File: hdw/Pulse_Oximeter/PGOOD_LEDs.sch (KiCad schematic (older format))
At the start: 8 parts

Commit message: Continued schematic development
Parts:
- removed C?: 0.1uF, Capacitors_SMD:C_0402, symbol Custom_Library:C_Custom
- removed D?: Green, LEDs:LED_0402, symbol Device:LED
- removed R?: 1k, Resistors_SMD:R_0402, symbol Custom_Library:R_Custom
- removed U?: 74LVC1G97, Package_TO_SOT_SMD:SOT-363_SC-70-6, symbol Custom_Library:74LVC1G97_Power_NOT
- added C? (x4): 0.1uF, Capacitors_SMD:C_0603, symbol Custom_Library:C_Custom
- added C?: 4.7uF, Capacitors_SMD:C_0805, symbol Custom_Library:C_Custom
- added D? (x4): Green, LEDs:LED_0603, symbol Device:LED
- added R? (x4): 1k, Resistors_SMD:R_0603, symbol Custom_Library:R_Custom
- added U? (x4): 74LVC1G97, Package_TO_SOT_SMD:SOT-363_SC-70-6, symbol Custom_Library:74LVC1G97_Power_NOT
- added U?: TPS71533, Package_TO_SOT_SMD:SOT-353_SC-70-5, symbol Regulator_Linear:TPS71533__SC70
- C?: footprint Capacitors_SMD:C_0402 -> Capacitors_SMD:C_0603; Digi-Key PN 490-10701-1-ND -> 311-1344-1-ND; display_footprint 0402 -> 0603
- D?: footprint LEDs:LED_0402 -> LEDs:LED_0603; Digi-Key PN 1497-1219-1-ND -> 160-1446-1-ND
- R?: footprint Resistors_SMD:R_0402 -> Resistors_SMD:R_0603; Digi-Key PN 541-1.00KLCT-ND -> RMCF0603FT1K00CT-ND; Wattage 1/16W -> 1/10W; display_footprint 0402 -> 0603
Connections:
- net labels added: +12V, POS12_PGOOD, POS1P8_PGOOD
- net labels removed: +5V_USB, GND_USB
- wire segments 4 -> 19
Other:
- moved on the sheet: C?, D?, R?

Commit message: Added display circuits
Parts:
- removed U? (x5): 74LVC1G97, Package_TO_SOT_SMD:SOT-363_SC-70-6, symbol Custom_Library:74LVC1G97_Power_NOT
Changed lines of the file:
@@
 EESchema Schematic File Version 4
+LIBS:Pulse_Oximeter-cache
 EELAYER 30 0
 EELAYER END
@@
 POS5_USB_PGOOD
 $Comp
-L Custom_Library:74LVC1G97_Power_NOT U?
-U 1 1 5E4A38CE
-P 4980 2870
-AR Path="/5CB7A8BC/5E4A38CE" Ref="U?"  Part="1"
-AR Path="/5CB7A8C3/5E4A38CE" Ref="U?"  Part="1"
-AR Path="/5EAE4ADE/5E4A38CE" Ref="U?"  Part="1"
-F 0 "U?" H 5040 3020 50  0000 L CNN
-F 1 "74LVC1G97" H 5040 2720 50  0000 L CNN
-F 2 "Package_TO_SOT_SMD:SOT-363_SC-70-6" H 5030 2870 50  0001 C CNN
-F 3 "http://www.ti.com/lit/ds/symlink/sn74lvc1g97.pdf" H 5030 2870 50  0001 C CNN
-F 4 "296-15582-1-ND" H 4980 2870 50  0001 C CNN "Digi-Key PN"
-	1    4980 2870
-	1    0    0    -1
-$EndComp
-$Comp
-L Custom_Library:74LVC1G97_Power_NOT U?
-U 1 1 5E4A4421
-P 6980 2870
-AR Path="/5CB7A8BC/5E4A4421" Ref="U?"  Part="1"
-AR Path="/5CB7A8C3/5E4A4421" Ref="U?"  Part="1"
-AR Path="/5EAE4ADE/5E4A4421" Ref="U?"  Part="1"
-F 0 "U?" H 7040 3020 50  0000 L CNN
-F 1 "74LVC1G97" H 7040 2720 50  0000 L CNN
-F 2 "Package_TO_SOT_SMD:SOT-363_SC-70-6" H 7030 2870 50  0001 C CNN
-F 3 "http://www.ti.com/lit/ds/symlink/sn74lvc1g97.pdf" H 7030 2870 50  0001 C CNN
-F 4 "296-15582-1-ND" H 6980 2870 50  0001 C CNN "Digi-Key PN"
-	1    6980 2870
-	1    0    0    -1
-$EndComp
-$Comp
-L Custom_Library:74LVC1G97_Power_NOT U?
-U 1 1 5E4A5210
-P 8980 2870
-AR Path="/5CB7A8BC/5E4A5210" Ref="U?"  Part="1"
-AR Path="/5CB7A8C3/5E4A5210" Ref="U?"  Part="1"
-AR Path="/5EAE4ADE/5E4A5210" Ref="U?"  Part="1"
-F 0 "U?" H 9040 3020 50  0000 L CNN
-F 1 "74LVC1G97" H 9040 2720 50  0000 L CNN
-F 2 "Package_TO_SOT_SMD:SOT-363_SC-70-6" H 9030 2870 50  0001 C CNN
-F 3 "http://www.ti.com/lit/ds/symlink/sn74lvc1g97.pdf" H 9030 2870 50  0001 C CNN
-F 4 "296-15582-1-ND" H 8980 2870 50  0001 C CNN "Digi-Key PN"
-	1    8980 2870
-	1    0    0    -1
-$EndComp
-$Comp
-L Custom_Library:74LVC1G97_Power_NOT U?
-U 1 1 5E4A7AA3
-P 2980 4370
-AR Path="/5CB7A8BC/5E4A7AA3" Ref="U?"  Part="1"
-AR Path="/5CB7A8C3/5E4A7AA3" Ref="U?"  Part="1"
-AR Path="/5EAE4ADE/5E4A7AA3" Ref="U?"  Part="1"
-F 0 "U?" H 3040 4520 50  0000 L CNN
-F 1 "74LVC1G97" H 3040 4220 50  0000 L CNN
-F 2 "Package_TO_SOT_SMD:SOT-363_SC-70-6" H 3030 4370 50  0001 C CNN
-F 3 "http://www.ti.com/lit/ds/symlink/sn74lvc1g97.pdf" H 3030 4370 50  0001 C CNN
-F 4 "296-15582-1-ND" H 2980 4370 50  0001 C CNN "Digi-Key PN"
-	1    2980 4370
-	1    0    0    -1
-$EndComp
-$Comp
 L Regulator_Linear:TPS71533__SC70 U?
 U 1 1 5E4D26A0
@@
 Wire Wire Line
 	2570 1950 2980 1950
-$Comp
-L Custom_Library:74LVC1G97_Power_NOT U?
-U 1 1 5E4A29B8
-P 2980 2870
-AR Path="/5CB7A8BC/5E4A29B8" Ref="U?"  Part="1"
-AR Path="/5CB7A8C3/5E4A29B8" Ref="U?"  Part="1"
-AR Path="/5EAE4ADE/5E4A29B8" Ref="U?"  Part="1"
-F 0 "U?" H 3040 3020 50  0000 L CNN
-F 1 "74LVC1G97" H 3040 2720 50  0000 L CNN
-F 2 "Package_TO_SOT_SMD:SOT-363_SC-70-6" H 3030 2870 50  0001 C CNN
-F 3 "http://www.ti.com/lit/ds/symlink/sn74lvc1g97.pdf" H 3030 2870 50  0001 C CNN
-F 4 "296-15582-1-ND" H 2980 2870 50  0001 C CNN "Digi-Key PN"
-	1    2980 2870
-	1    0    0    -1
-$EndComp
 $EndSCHEMATC

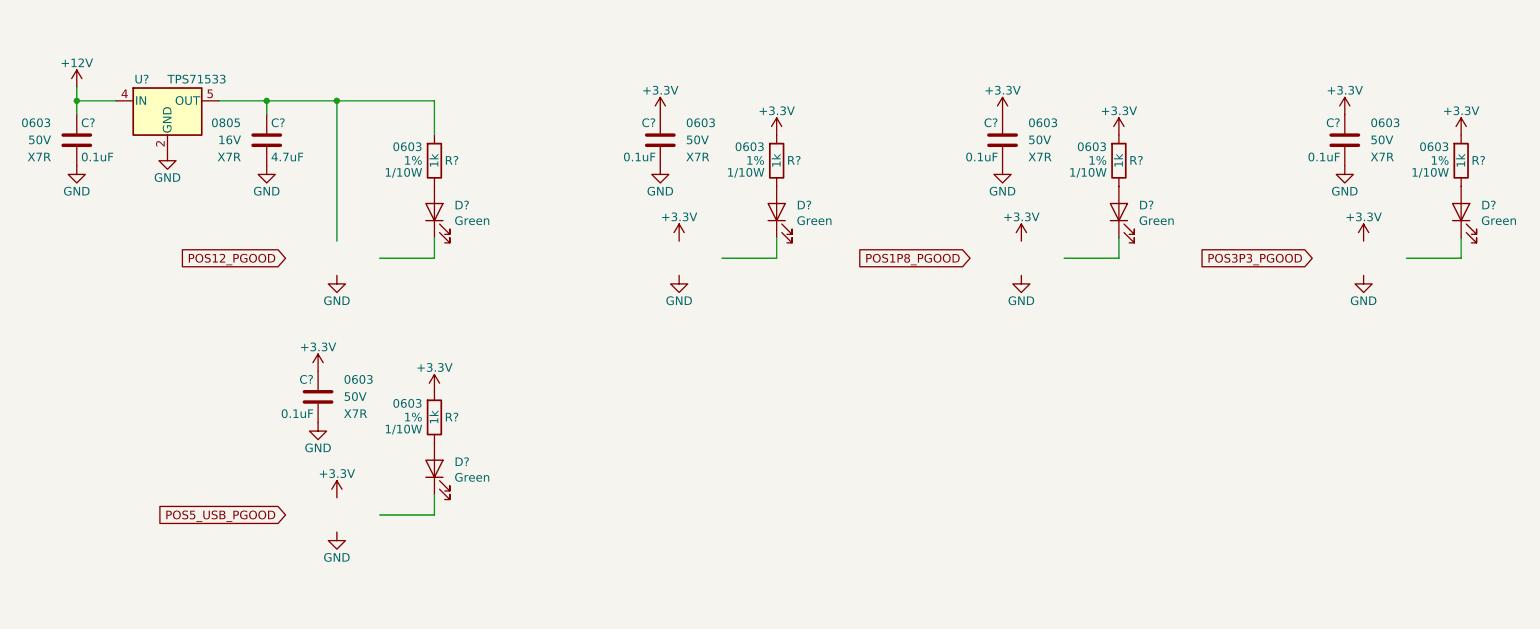
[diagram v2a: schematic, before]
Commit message: few sch additions
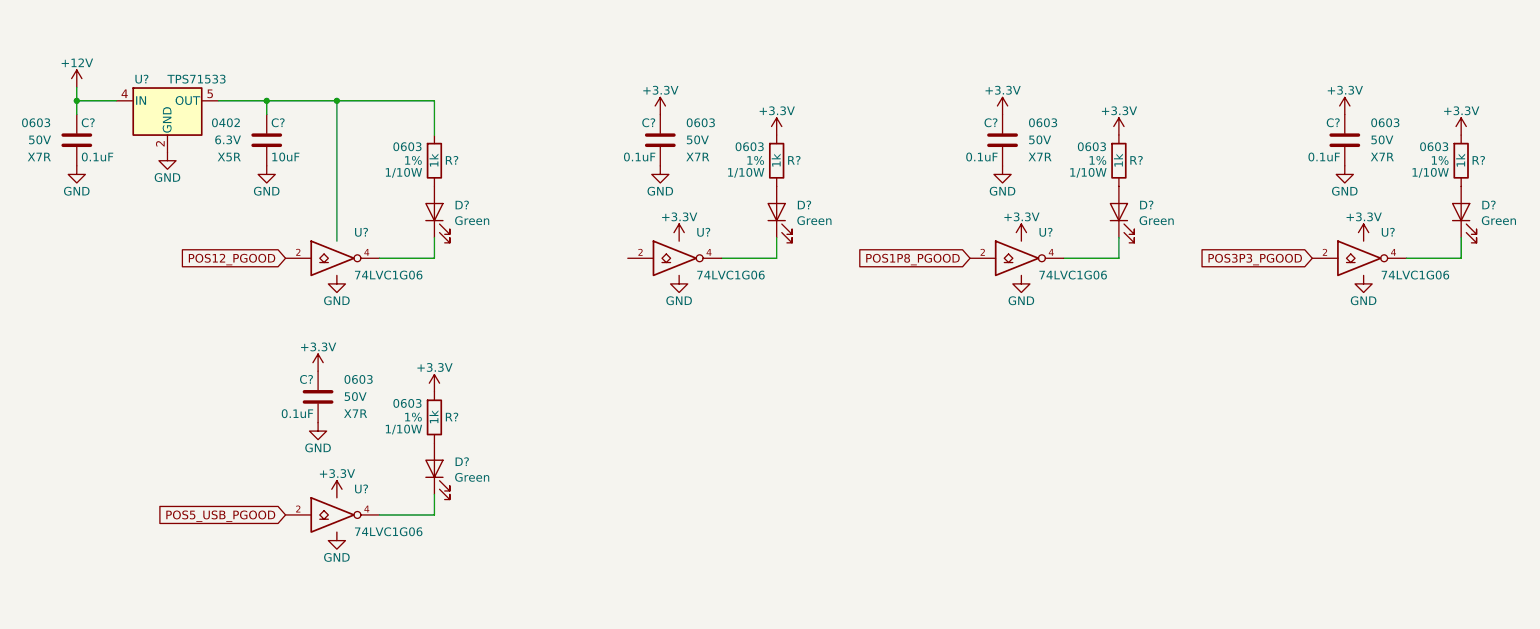
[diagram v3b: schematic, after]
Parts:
- removed C?: 4.7uF, Capacitors_SMD:C_0805, symbol Custom_Library:C_Custom
- added C?: 10uF, Capacitors_SMD:C_0402, symbol Custom_Library:C_Custom
- added U? (x5): 74LVC1G06, TO_SOT_Packages_SMD:SOT-353_SC-70-5, symbol Custom_Library:74LVC1G06_Power
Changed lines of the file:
@@
-$Comp
-L Custom_Library:C_Custom C?
-U 1 1 5E1765D3
-P 2570 2180
-AR Path="/5A0BC776/5E1765D3" Ref="C?"  Part="1"
-AR Path="/5CB7A8C3/5E1765D3" Ref="C?"  Part="1"
-AR Path="/5EAE4ADE/5E1765D3" Ref="C?"  Part="1"
-F 0 "C?" H 2595 2280 50  0000 L CNN
-F 1 "4.7uF" H 2595 2080 50  0000 L CNN
-F 2 "Capacitors_SMD:C_0805" H 2608 2030 50  0001 C CNN
-F 3 "" H 2595 2280 50  0001 C CNN
-F 4 "0805" H 2420 2280 50  0000 R CNN "display_footprint"
-F 5 "16V" H 2420 2180 50  0000 R CNN "Voltage"
-F 6 "X7R" H 2420 2080 50  0000 R CNN "Dielectric"
-F 7 "1276-2970-1-ND" H -3330 -2380 50  0001 C CNN "Digi-Key PN"
-	1    2570 2180
-	1    0    0    -1
-$EndComp
 $Comp
 L Custom_Library:C_Custom C?
@@
 Wire Wire Line
 	2570 1950 2980 1950
+$Comp
+L Custom_Library:74LVC1G06_Power U?
+U 1 1 5EBA890C
+P 2980 2870
+F 0 "U?" H 3080 3020 50  0000 L CNN
+F 1 "74LVC1G06" H 3080 2770 50  0000 L CNN
+F 2 "TO_SOT_Packages_SMD:SOT-353_SC-70-5" H 2980 2920 50  0001 C CNN
+F 3 "http://www.ti.com/lit/ds/symlink/sn74lvc1g06.pdf" H 2980 2870 50  0001 C CNN
+F 4 "296-8484-1-ND" H 2980 2870 50  0001 C CNN "Digi-Key PN"
+	1    2980 2870
+	1    0    0    -1
+$EndComp
+$Comp
+L Custom_Library:74LVC1G06_Power U?
+U 1 1 5EBAD160
+P 4980 2870
+F 0 "U?" H 5080 3020 50  0000 L CNN
+F 1 "74LVC1G06" H 5080 2770 50  0000 L CNN
+F 2 "TO_SOT_Packages_SMD:SOT-353_SC-70-5" H 4980 2920 50  0001 C CNN
+F 3 "http://www.ti.com/lit/ds/symlink/sn74lvc1g06.pdf" H 4980 2870 50  0001 C CNN
+F 4 "296-8484-1-ND" H 4980 2870 50  0001 C CNN "Digi-Key PN"
+	1    4980 2870
+	1    0    0    -1
+$EndComp
+$Comp
+L Custom_Library:74LVC1G06_Power U?
+U 1 1 5EBADD05
+P 6980 2870
+F 0 "U?" H 7080 3020 50  0000 L CNN
+F 1 "74LVC1G06" H 7080 2770 50  0000 L CNN
+F 2 "TO_SOT_Packages_SMD:SOT-353_SC-70-5" H 6980 2920 50  0001 C CNN
+F 3 "http://www.ti.com/lit/ds/symlink/sn74lvc1g06.pdf" H 6980 2870 50  0001 C CNN
+F 4 "296-8484-1-ND" H 6980 2870 50  0001 C CNN "Digi-Key PN"
+	1    6980 2870
+	1    0    0    -1
+$EndComp
+$Comp
+L Custom_Library:74LVC1G06_Power U?
+U 1 1 5EBAE6FA
+P 8980 2870
+F 0 "U?" H 9080 3020 50  0000 L CNN
+F 1 "74LVC1G06" H 9080 2770 50  0000 L CNN
+F 2 "TO_SOT_Packages_SMD:SOT-353_SC-70-5" H 8980 2920 50  0001 C CNN
+F 3 "http://www.ti.com/lit/ds/symlink/sn74lvc1g06.pdf" H 8980 2870 50  0001 C CNN
+F 4 "296-8484-1-ND" H 8980 2870 50  0001 C CNN "Digi-Key PN"
+	1    8980 2870
+	1    0    0    -1
+$EndComp
+$Comp
+L Custom_Library:74LVC1G06_Power U?
+U 1 1 5EBAEFAB
+P 2980 4370
+F 0 "U?" H 3080 4520 50  0000 L CNN
+F 1 "74LVC1G06" H 3080 4270 50  0000 L CNN
+F 2 "TO_SOT_Packages_SMD:SOT-353_SC-70-5" H 2980 4420 50  0001 C CNN
+F 3 "http://www.ti.com/lit/ds/symlink/sn74lvc1g06.pdf" H 2980 4370 50  0001 C CNN
+F 4 "296-8484-1-ND" H 2980 4370 50  0001 C CNN "Digi-Key PN"
+	1    2980 4370
+	1    0    0    -1
+$EndComp
+$Comp
+L Custom_Library:C_Custom C?
+U 1 1 5EBBADED
+P 2570 2180
+AR Path="/5CB7718D/5EBBADED" Ref="C?"  Part="1"
+AR Path="/5E0DC082/5EBBADED" Ref="C?"  Part="1"
+AR Path="/5E0F9110/5EBBADED" Ref="C?"  Part="1"
+AR Path="/5A557C58/5EBBADED" Ref="C?"  Part="1"
+AR Path="/5CB25152/5EBBADED" Ref="C?"  Part="1"
+AR Path="/5E697934/5EBBADED" Ref="C?"  Part="1"
+AR Path="/5EAE2F02/5EBBADED" Ref="C?"  Part="1"
+AR Path="/5EAE3021/5EBBADED" Ref="C?"  Part="1"
+AR Path="/5EAE4ADE/5EBBADED" Ref="C?"  Part="1"
+F 0 "C?" H 2595 2280 50  0000 L CNN
+F 1 "10uF" H 2595 2080 50  0000 L CNN
+F 2 "Capacitors_SMD:C_0402" H 2608 2030 50  0001 C CNN
+F 3 "" H 2595 2280 50  0001 C CNN
+F 4 "0402" H 2420 2280 50  0000 R CNN "display_footprint"
+F 5 "6.3V" H 2420 2180 50  0000 R CNN "Voltage"
+F 6 "X5R" H 2420 2080 50  0000 R CNN "Dielectric"
+F 7 "490-13211-1-ND" H 2570 2180 50  0001 C CNN "Digi-Key PN"
+	1    2570 2180
+	1    0    0    -1
+$EndComp
 $EndSCHEMATC
